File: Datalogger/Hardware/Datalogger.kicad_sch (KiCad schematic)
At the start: 22 parts, among them J1 SD_Card, J2 Conn_01x03_Pin, J3 Conn_01x03_Pin, SW1 SW_Push, SW2 SW_SPST, U1 STM32F042F6Px, U2 LM1117DT-3.3, U3 MCP2562-E-SN

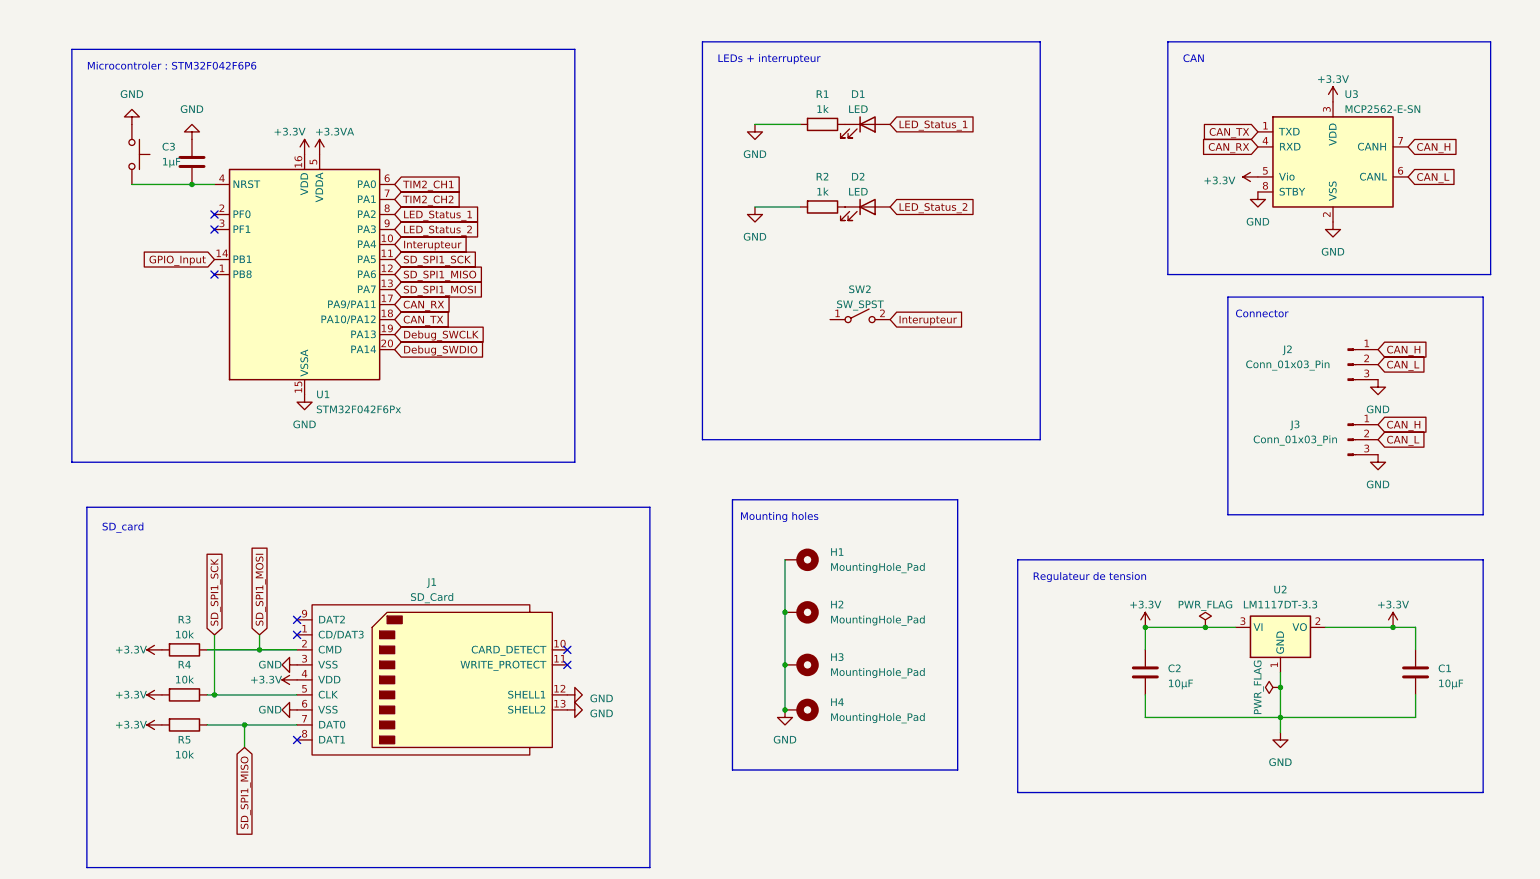
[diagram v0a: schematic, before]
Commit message: Kikad Sch ok
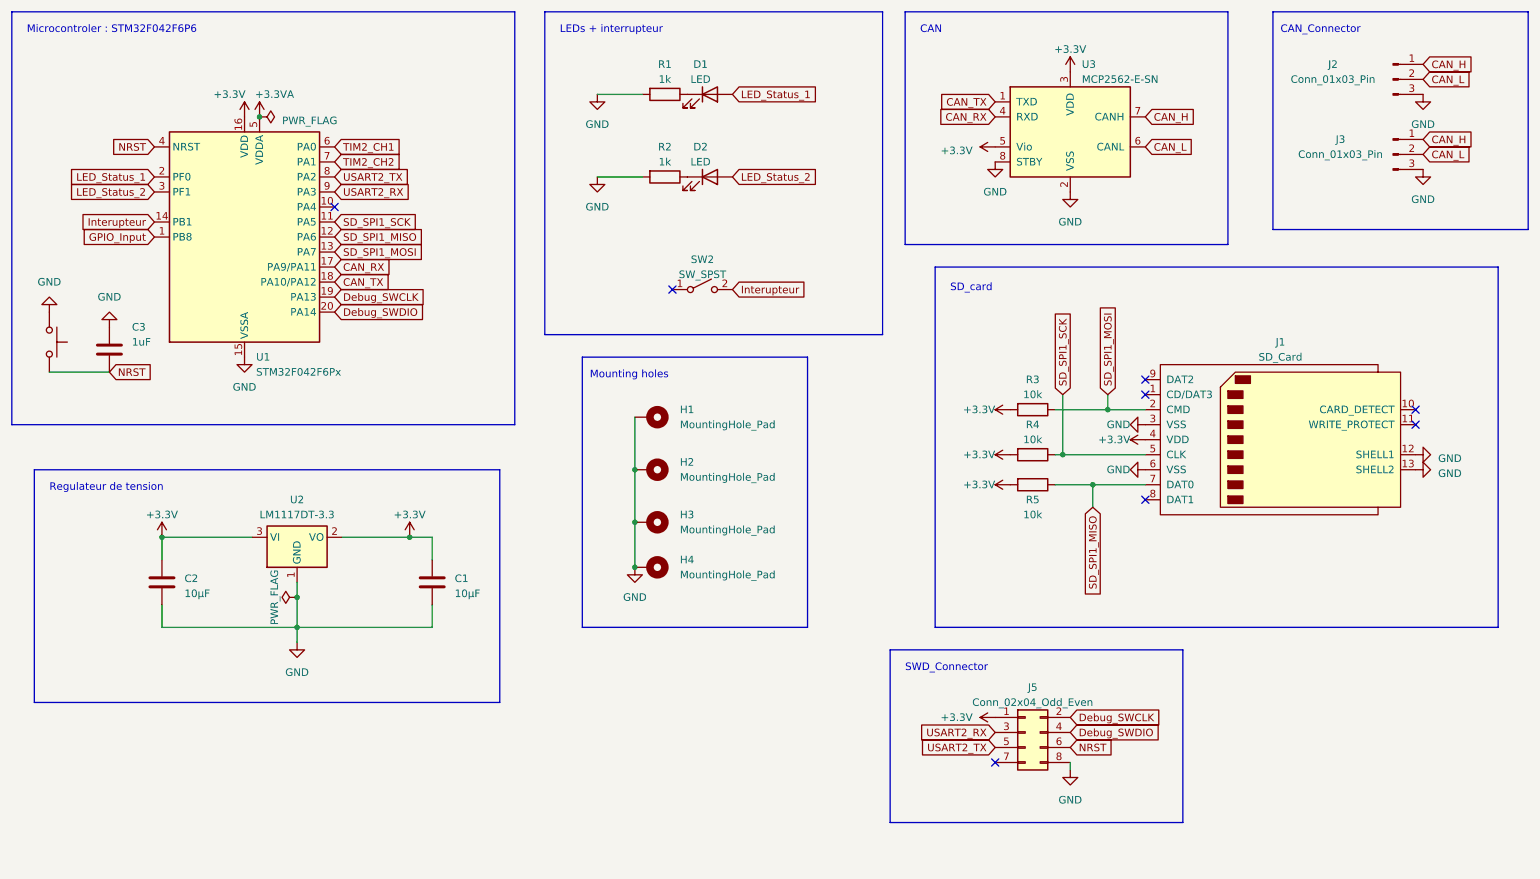
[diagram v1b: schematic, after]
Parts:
- added J5: Conn_02x04_Odd_Even, symbol Connector_Generic:Conn_02x04_Odd_Even
- C1, C2: footprint Capacitor_SMD:C_0805_2012Metric_Pad1.18x1.45mm_HandSolder -> (none)
- C3: value 1µF -> 1uF; footprint Capacitor_SMD:C_0805_2012Metric_Pad1.18x1.45mm_HandSolder -> (none)
- D1, D2: footprint Diode_SMD:D_0201_0603Metric_Pad0.64x0.40mm_HandSolder -> (none)
- H1, H2, H3, H4: footprint MountingHole:MountingHole_2.2mm_M2_DIN965_Pad -> (none)
- R1, R2, R3, R4, R5: footprint Resistor_SMD:R_0603_1608Metric_Pad0.98x0.95mm_HandSolder -> (none)
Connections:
- net +3.3V: now also J5.1 (Pin_1)
- net Debug_SWCLK: now also J5.2 (Pin_2)
- net Debug_SWDIO: now also J5.4 (Pin_4)
- net GND: now also C3.1, J5.8 (Pin_8); no longer C3.2
- net GPIO_Input: now also U1.1 (PB8); no longer U1.14 (PB1)
- net Interupteur: now also U1.14 (PB1); no longer U1.10 (PA4)
- net LED_Status_1: now also U1.2 (PF0); no longer U1.8 (PA2)
- net LED_Status_2: now also U1.3 (PF1); no longer U1.9 (PA3)
- net NRST: now reaches SW1.2, U1.4 (NRST)
- net NRST: now also C3.2, J5.6 (Pin_6); no longer C3.1
- new net USART2_RX: J5.3 (Pin_3), U1.9 (PA3)
- new net USART2_TX: J5.5 (Pin_5), U1.8 (PA2)
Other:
- note added: "CAN_Connector"
- note added: "SWD_Connector"
- note removed: "Connector"
- moved on the sheet: C1, C2, D1, D2, H1, H2, H3, H4, J1, J2, J3, R1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
